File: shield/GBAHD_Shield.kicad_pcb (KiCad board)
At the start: 2 copper layers, 53.4 x 53.1 mm, 38 parts, among them J1 Conn_01x01, J10 Conn_01x10, J11 Conn_02x03_Odd_Even, J12 Conn_01x01, J2 FFC_OGBA_32, J3 FFC_GBA-SP, J4 Conn_01x16, J5 FFC_OGBA_40, J6 Conn_01x06, J7 Conn_01x08, J8 Conn_01x10, J9 Conn_01x08, Q1 Q_PMOS_GSD, SW1 SW_Push, T1 Conn_01x01, T2 Conn_01x01, T3 Conn_01x01, T4 Conn_01x01, T5 Conn_01x01, T6 Conn_01x01, T7 Conn_01x01, T8 Conn_01x01, U1 AZ1117R-ADJ, U2 74HC595, U3 74HC595, U4 SNES_7PIN, U5 ATmega328P-AU

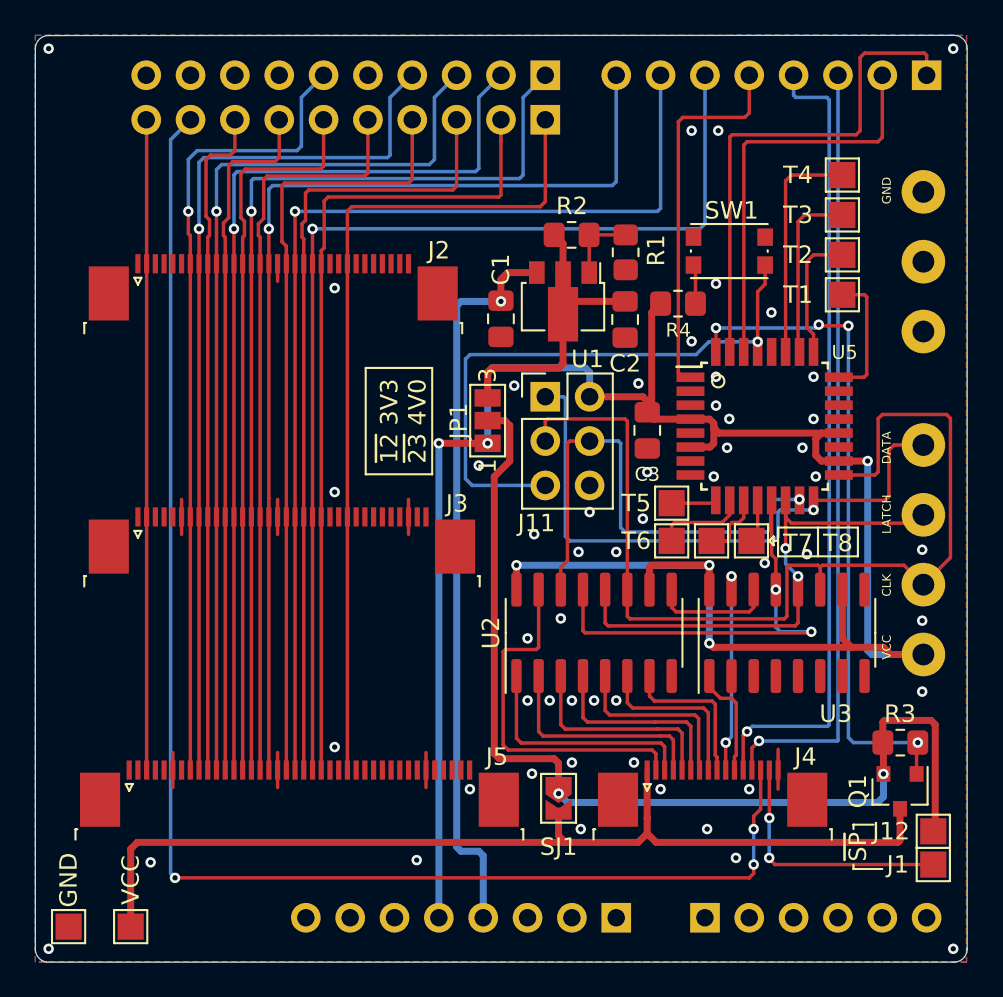
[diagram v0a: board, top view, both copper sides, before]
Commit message: updated shield
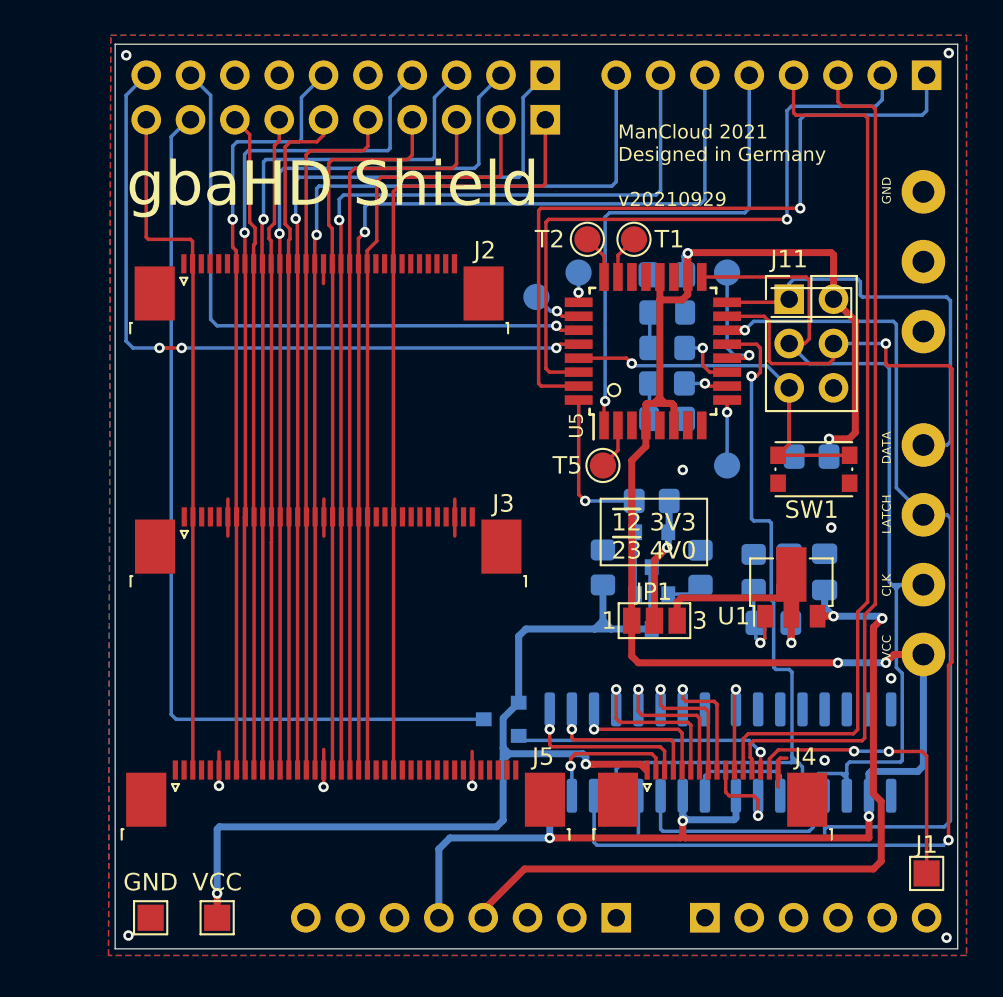
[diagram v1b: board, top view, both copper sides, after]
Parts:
- removed J12, T8: Conn_01x01, TestPoint:TestPoint_Pad_1.5x1.5mm
- removed SJ1: SOLDER_JUMPER, Jumper:SolderJumper-2_P1.3mm_Open_TrianglePad1.0x1.5mm
- added D1: RED, LED_SMD:LED_0805_2012Metric_Pad1.15x1.40mm_HandSolder, B.Cu at (75.8, 48.4)
- added D2: GREEN, LED_SMD:LED_0805_2012Metric_Pad1.15x1.40mm_HandSolder, B.Cu at (75.8, 42.3)
- added Q2: Q_NMOS_GSD, Package_TO_SOT_SMD:SOT-23, B.Cu at (74.9, 59.4)
- added Q3: Q_NMOS_GSD, Package_TO_SOT_SMD:SOT-23, B.Cu at (66.3, 65.6)
- added R5: 500, Resistor_SMD:R_0805_2012Metric_Pad1.20x1.40mm_HandSolder, B.Cu at (77.7, 56.9)
- added R6: 10K, Resistor_SMD:R_0805_2012Metric_Pad1.20x1.40mm_HandSolder, B.Cu at (75.8, 46.4)
- added R7: 10K, Resistor_SMD:R_0805_2012Metric_Pad1.20x1.40mm_HandSolder, B.Cu at (75.8, 44.3)
- added R8: 10K, Resistor_SMD:R_0805_2012Metric_Pad1.20x1.40mm_HandSolder, B.Cu at (72.1, 56.9)
- C1, C2, C3, Q1, R1, R2, R3, R4, U2, U3: moved to B.Cu
- T1, T2, T5: footprint TestPoint:TestPoint_Pad_1.5x1.5mm -> TestPoint:TestPoint_Pad_D1.5mm
- T3, T4, T6, T7: footprint TestPoint:TestPoint_Pad_1.5x1.5mm -> TestPoint:TestPoint_Pad_D1.5mm; moved to B.Cu
- moved R2 25.1 mm to (81.9, 60.1), turned to 0 degrees
- moved C1 23.5 mm to (84.8, 57.1), turned to 270 degrees
- moved U1 21.0 mm to (82.9, 58.0), turned to 90 degrees
- moved R3 19.9 mm to (74.9, 53.1), turned to 0 degrees
- moved Q1 19.8 mm to (74.9, 55.9)
- moved R1 19.7 mm to (80.8, 57.1), turned to 270 degrees
- moved T4 18.9 mm to (68.3, 41.4)
- moved C2 17.2 mm to (82.8, 57.1), turned to 270 degrees
- moved T3 15.5 mm to (70.7, 40.0)
- moved T7 15.4 mm to (79.2, 40.0)
- moved J11 15.0 mm to (82.8, 41.5)
- moved JP1 14.9 mm to (75.1, 59.9), turned to 0 degrees
- moved T2 14.6 mm to (71.2, 38.1)
- moved SW1 13.4 mm to (84.2, 51.3), turned to 0 degrees
- moved T1 12.4 mm to (73.9, 38.1)
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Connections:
- net PIXEL_GRID renamed FPGA_COM
- J10 pad 10: (no net) -> SP_ARSCL
- J10 pad 9: (no net) -> SP_ARSDA
- J4 pad 14: GBA_CLK -> GBA_CLK'
- U5 pad 10: Net-(T6-Pad1) -> LED_RED
- U5 pad 11: Net-(T7-Pad1) -> LED_GREEN
- U5 pad 12: Net-(T8-Pad1) -> Net-(T7-Pad1)
- U5 pad 2: (no net) -> Net-(T5-Pad1)
- U5 pad 23: (no net) -> Net-(T1-Pad1)
- U5 pad 24: Net-(T1-Pad1) -> Net-(T2-Pad1)
- U5 pad 25: Net-(T2-Pad1) -> Net-(T3-Pad1)
- U5 pad 26: Net-(T3-Pad1) -> Net-(T4-Pad1)
- U5 pad 27: Net-(T4-Pad1) -> SP_ARSDA
- U5 pad 28: (no net) -> SP_ARSCL
- U5 pad 9: Net-(T5-Pad1) -> Net-(T6-Pad1)
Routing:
- net VCC: track 57.9 -> 7.21 mm, vias 2 -> 1
- net SP_ARSCL: track 0.00 -> 41.9 mm, vias 0 -> 3
- net ICSP_MOSI: track 28.6 -> 67.9 mm, vias 1 -> 2
- net SP_ARSDA: track 0.00 -> 35.8 mm, vias 0 -> 1
- net SNS_LATCH: track 29.7 -> 63.4 mm, vias 2 -> 1
- net GBA_CLK: track 83.3 -> 52.6 mm, vias 3 -> 0
- net GBA_POWER_SEL: track 38.6 -> 14.1 mm, vias 4 -> 1
- net ~GBA_BUTTONS_EN~: track 25.0 -> 42.7 mm, vias 2 -> 1
- net GBA_CLK': track 0.00 -> 15.3 mm, vias 0 -> 1
- net SP_ARD1: track 23.6 -> 37.6 mm, vias 0 -> 1
- net GBA_UP: track 20.7 -> 7.95 mm, vias 0 -> 1
- net RX: track 29.3 -> 41.9 mm, vias 0 -> 1
- net AT_RST: track 36.1 -> 25.0 mm
- net Net-(T4-Pad1): track 13.2 -> 2.88 mm, vias 0 -> 1
- net ICSP_MISO: track 34.1 -> 24.5 mm, vias 1 -> 0
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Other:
- board size 53.4 x 53.1 mm -> 48.3 x 51.8 mm
- board text added: "ManCloud 2021 Designed in Germany v20210929"
- board text removed: "ManCloud 2021 Designed in Germany v20210416"
- board text removed: "~SP~"
